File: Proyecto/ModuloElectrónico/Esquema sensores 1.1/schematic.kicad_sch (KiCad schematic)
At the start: 30 parts, among them J1 DO-IN, J2 TEMP_IN, J3 PH_IN, J4 TURB_IN, U1 Opamp_Dual, U2 Opamp_Quad, U3 Opamp_Quad

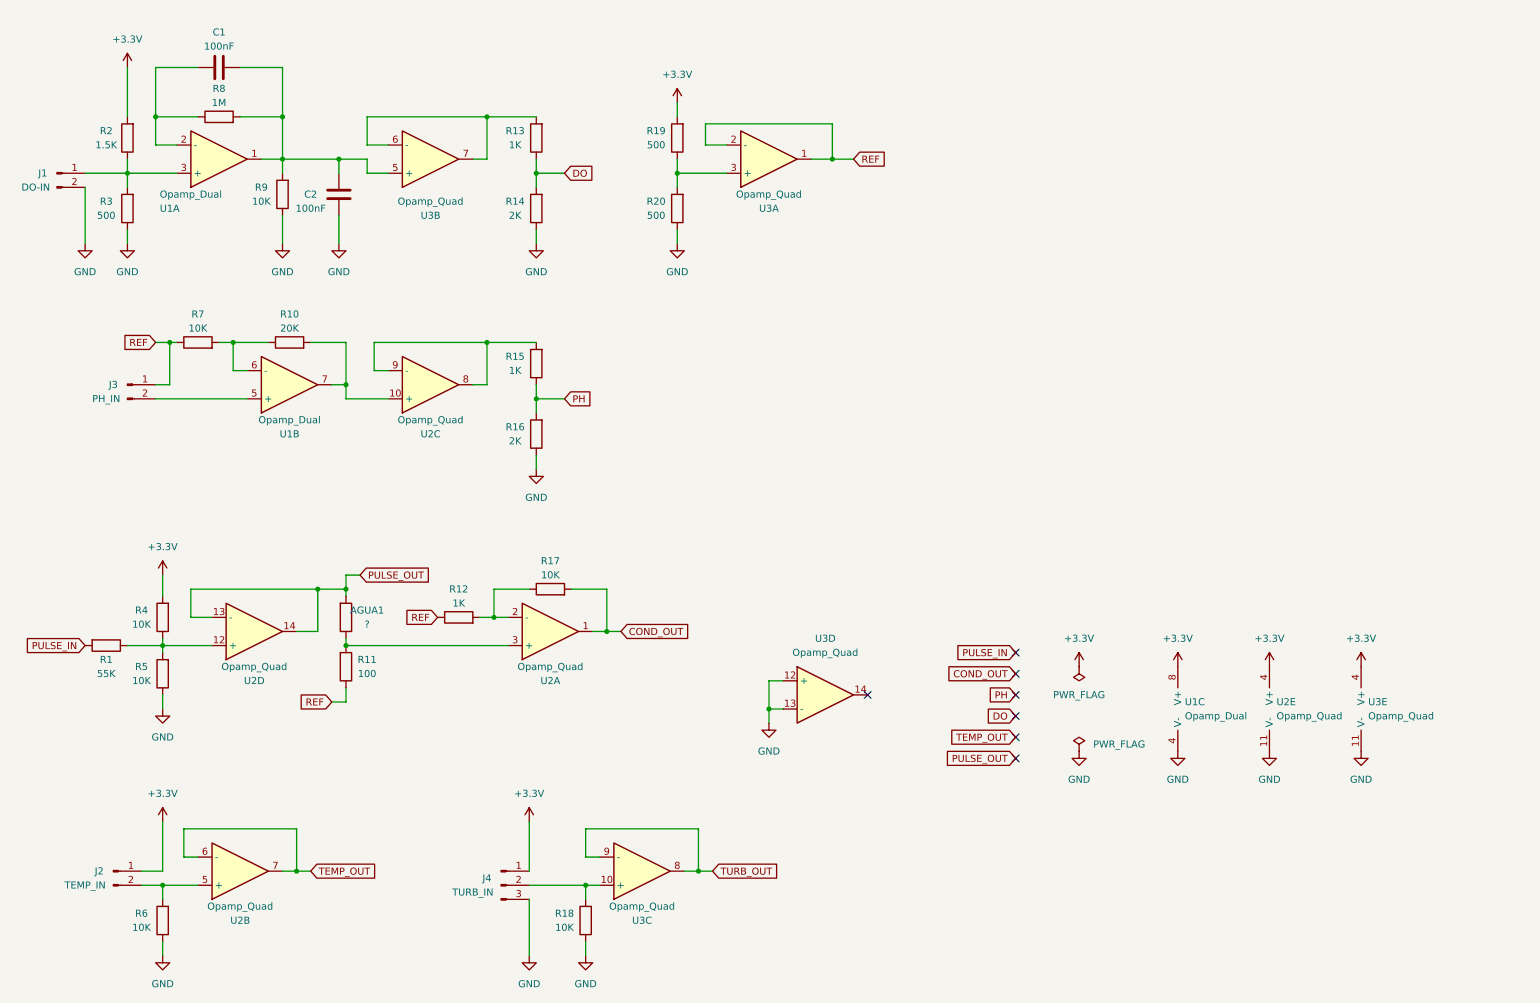
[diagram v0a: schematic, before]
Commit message: Actualización de archivos
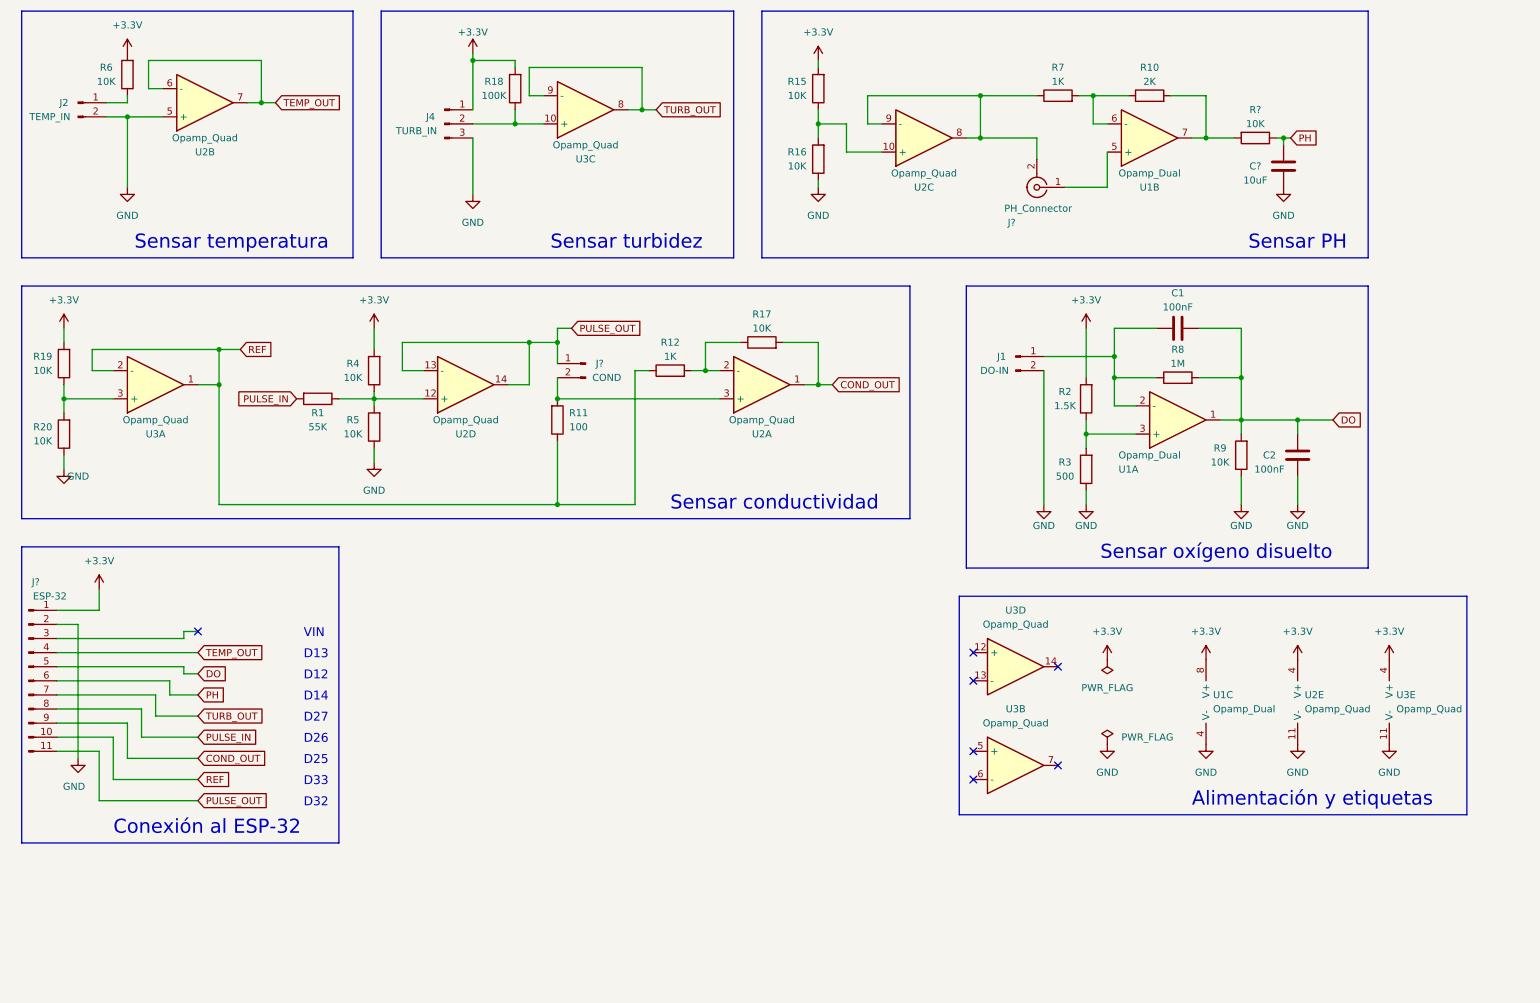
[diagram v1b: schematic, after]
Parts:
- removed AGUA1: ?, symbol Device:R
- removed J3: PH_IN, symbol Connector:Conn_01x02_Male
- removed R13: 1K, symbol Device:R
- removed R14: 2K, symbol Device:R
- added C?: 10uF, symbol Device:C
- added J?: ESP-32, symbol Connector:Conn_01x11_Male
- added J?: COND, symbol Connector:Conn_01x02_Male
- added J?: PH_Connector, symbol Connector:Conn_Coaxial
- added R?: 10K, symbol Device:R
- R10: value 20K -> 2K
- R15: value 1K -> 10K
- R16: value 2K -> 10K
- R18: value 10K -> 100K
- R19, R20: value 500 -> 10K
- R7: value 10K -> 1K
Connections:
- net +3.3V: now also R15.2, R18.2, R6.2, J?.1 (Pin_1); no longer J2.1 (Pin_1)
- net COND_OUT: now also J?.9 (Pin_9)
- net DO: now also C1.2, C2.2, R8.2, R9.2, U1.1, J?.5 (Pin_5)
- net GND: now also J2.2 (Pin_2), U2.5 (+), C?.1, J?.2 (Pin_2); no longer R18.1, R6.1, U3.12 (+), U3.13 (-)
- net PH: now also C?.2, J?.6 (Pin_6), R?.1; no longer R15.1, R16.2
- net PULSE_IN: now also J?.8 (Pin_8)
- net PULSE_OUT: now also J?.1 (Pin_1), J?.11 (Pin_11)
- net REF: now also J?.10 (Pin_10); no longer R7.1
- net TEMP_OUT: now also J?.4 (Pin_4)
- net TURB_OUT: now also J?.7 (Pin_7)
- net at R2.1, R3.2, U1.3 (+): no longer J1.1 (Pin_1)
- net at R11.2, U2.3 (+): now also J?.2 (Pin_2)
- net at C1.1, R8.1, U1.2 (-): now also J1.1 (Pin_1)
- net at J4.2 (Pin_2), U3.10 (+): now also R18.1; no longer R18.2
- net at U2.8, U2.9 (-): now also R7.1, J?.2 (Ext); no longer R15.2
- net at U3.6 (-): no longer U3.7
- net at R10.2, U1.7: now also R?.2; no longer U2.10 (+)
- net at U1.5 (+): now also J?.1 (In)
- new net: J2.1 (Pin_1), R6.1
- new net: R15.1, R16.2, U2.10 (+)
- now unconnected: U3.5 (+)
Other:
- note added: "Alimentación y etiquetas"
- note added: "Conexión al ESP-32"
- note added: "D12"
- note added: "D13"
- note added: "D14"
- note added: "D25"
- note added: "D26"
- note added: "D27"
- note added: "D32"
- note added: "D33"
- note added: "Sensar PH"
- note added: "Sensar conductividad"
- note added: "Sensar oxígeno disuelto"
- note added: "Sensar temperatura"
- note added: "Sensar turbidez"
- note added: "VIN"
- company: (none) -> UPCH-FDD-G10-DJWZ
- title: (none) -> Panel de sensores - EcoAqua
- moved on the sheet: C1, C2, J1, J2, J4, R1, R10, R11, R12, R15, R16, R17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
